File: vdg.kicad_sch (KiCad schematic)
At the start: 4 parts, among them IC12 MC6847, IC13 74LS273N

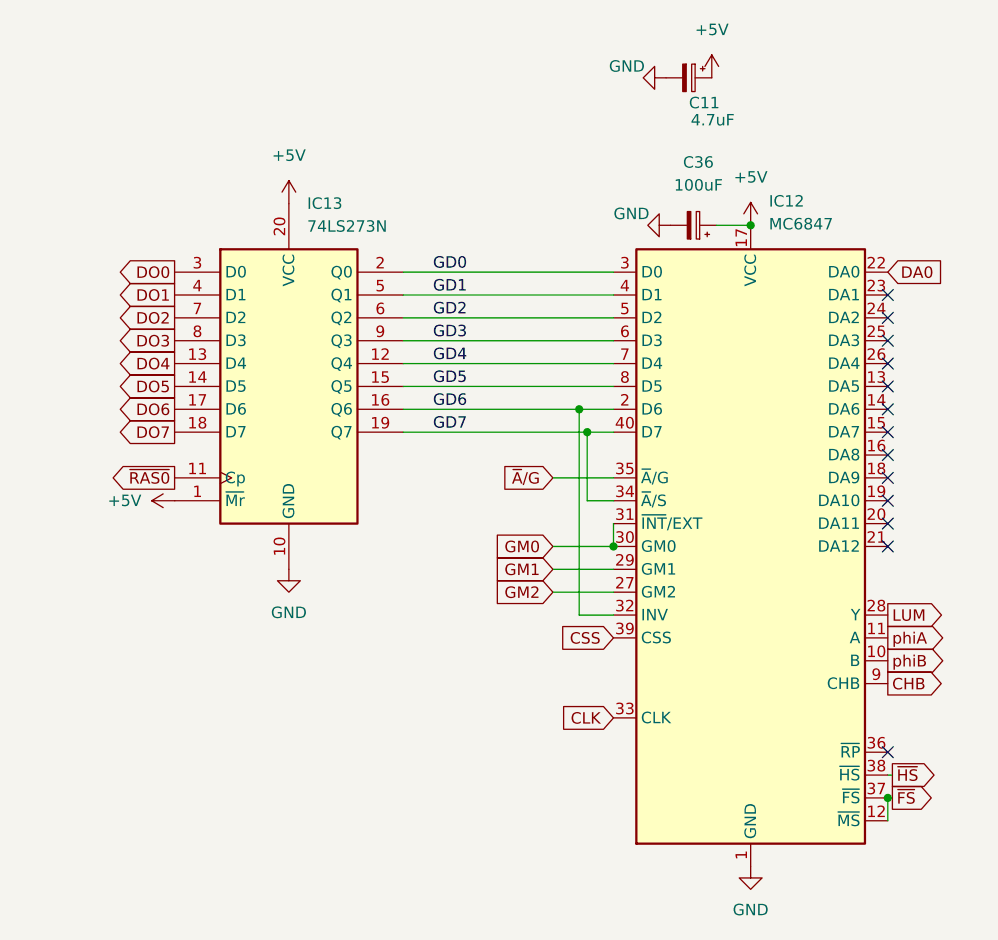
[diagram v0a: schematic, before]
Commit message: video circuit tracing
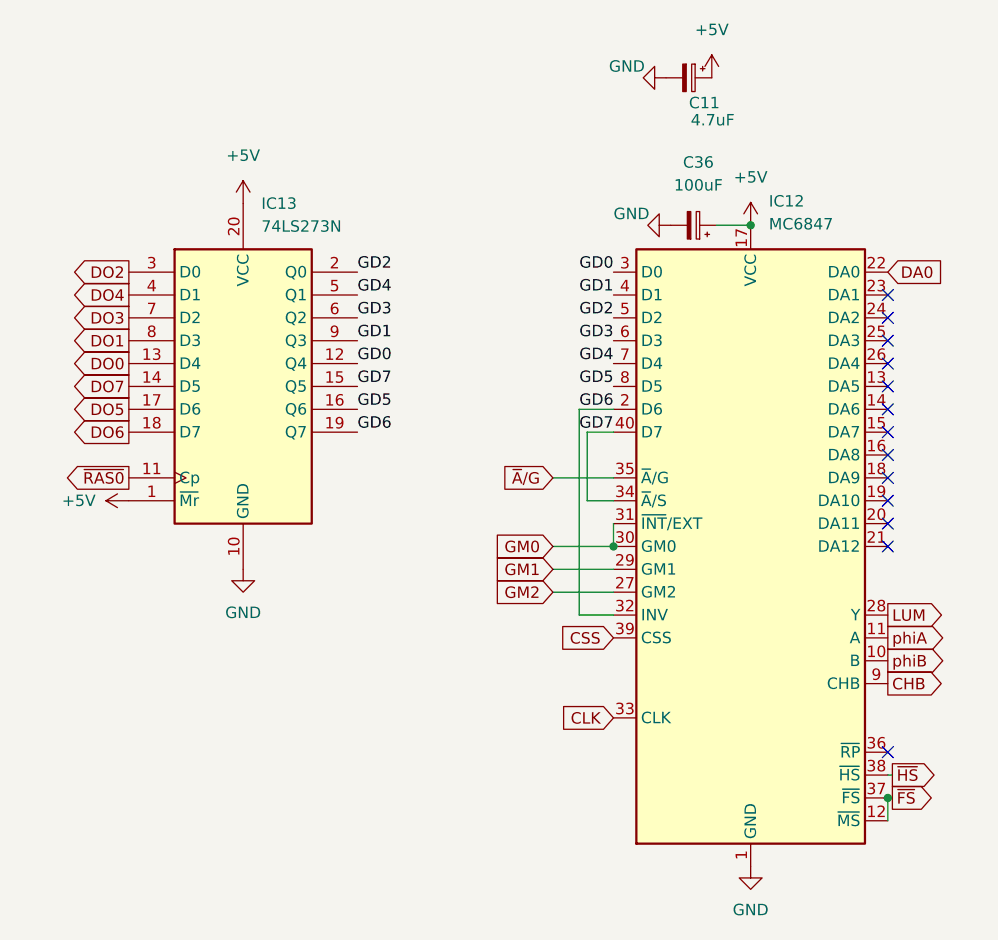
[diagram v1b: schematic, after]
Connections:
- net DO0: now also IC13.13 (D4); no longer IC13.3 (D0)
- net DO1: now also IC13.8 (D3); no longer IC13.4 (D1)
- net DO2: now also IC13.3 (D0); no longer IC13.7 (D2)
- net DO3: now also IC13.7 (D2); no longer IC13.8 (D3)
- net DO4: now also IC13.4 (D1); no longer IC13.13 (D4)
- net DO5: now also IC13.17 (D6); no longer IC13.14 (D5)
- net DO6: now also IC13.18 (D7); no longer IC13.17 (D6)
- net DO7: now also IC13.14 (D5); no longer IC13.18 (D7)
- net GD0: now also IC13.12 (Q4); no longer IC13.2 (Q0)
- net GD1: now also IC13.9 (Q3); no longer IC13.5 (Q1)
- net GD2: now also IC13.2 (Q0); no longer IC13.6 (Q2)
- net GD3: now also IC13.6 (Q2); no longer IC13.9 (Q3)
- net GD4: now also IC13.5 (Q1); no longer IC13.12 (Q4)
- net GD5: now also IC13.16 (Q6); no longer IC13.15 (Q5)
- net GD6: now also IC13.19 (Q7); no longer IC13.16 (Q6)
- net GD7: now also IC13.15 (Q5); no longer IC13.19 (Q7)
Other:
- moved on the sheet: IC13
